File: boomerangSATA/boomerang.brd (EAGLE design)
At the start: 84.1 x 79.3 mm, 12 parts

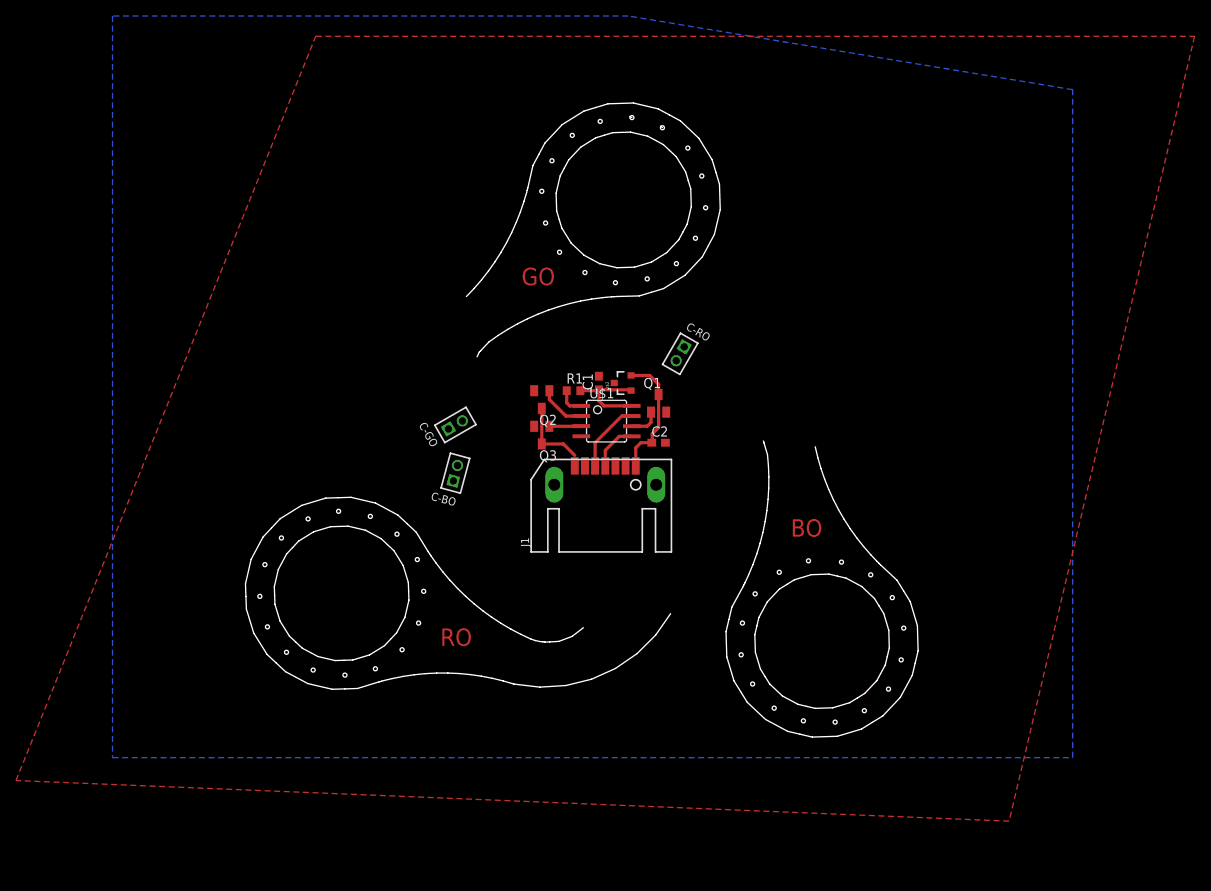
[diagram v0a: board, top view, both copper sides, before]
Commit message: foo
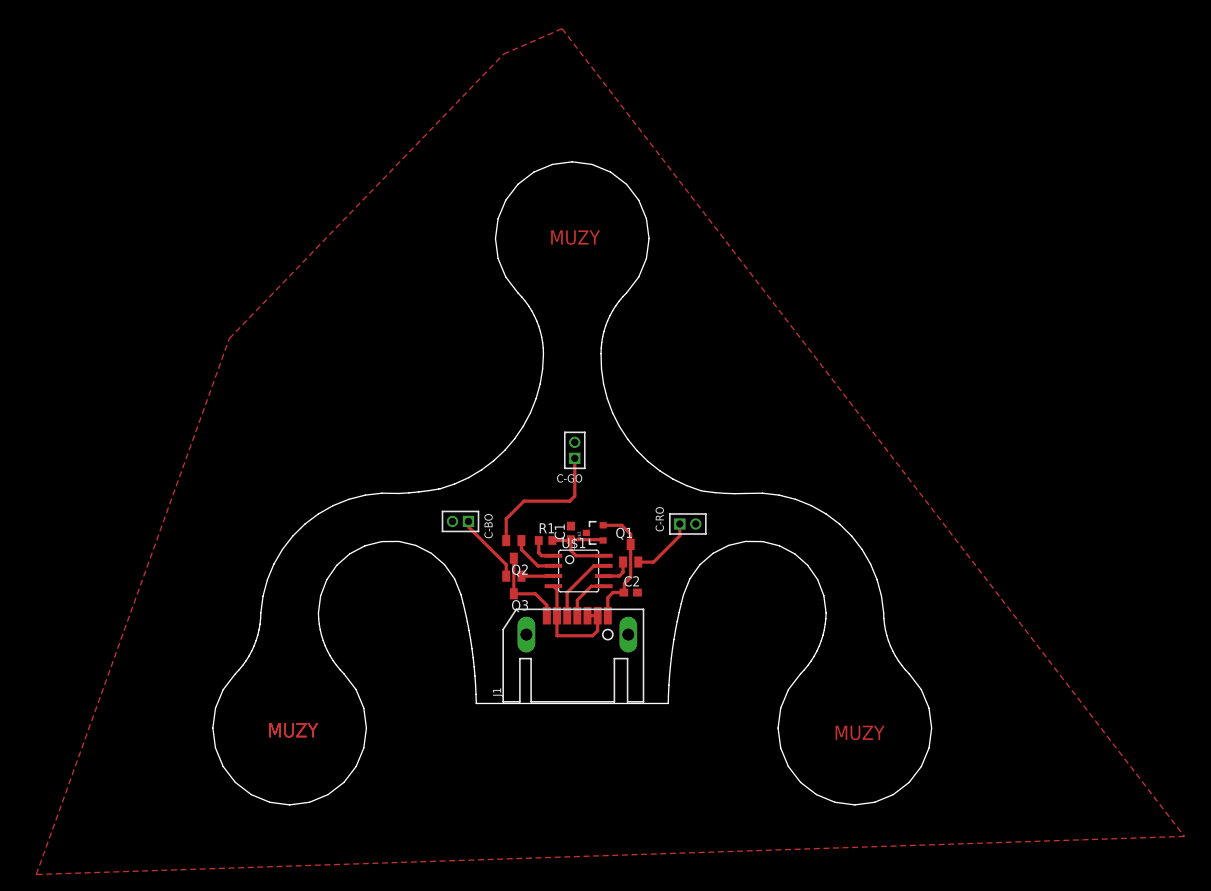
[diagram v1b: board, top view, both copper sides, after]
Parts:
- moved C-RO 21.3 mm to (14.4, -5.08), turned to 0 degrees
- moved C1 19.1 mm to (-0.16, -6.19)
- moved C2 19.1 mm to (7.30, -13.7)
- moved Q1 19.1 mm to (7.30, -8.73)
- moved Q2 19.1 mm to (-7.30, -8.26)
- moved U$2 19.1 mm to (2.86, -6.19)
- moved J1 19.1 mm to (0.64, -21.0)
- moved Q3 19.1 mm to (-7.30, -12.7)
- moved R1 19.1 mm to (-3.33, -7.14)
- moved U$1 19.1 mm to (0.79, -11.0)
- moved C-GO 15.3 mm to (0.32, 4.13), turned to 90 degrees
- moved C-BO 6.07 mm to (-14.0, -4.76), turned to 180 degrees
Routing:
- net GO: track 0.00 -> 17.2 mm
- net GND: track 0.00 -> 15.5 mm
- net BO: track 0.00 -> 8.86 mm
- net RO: track 0.00 -> 8.04 mm
- net VCC: track 25.3 -> 26.6 mm
- removed copper zone on layer 16, net GND
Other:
- board size 84.1 x 79.3 mm -> 89.8 x 80.4 mm
- board text added: "MUZY"
- board text removed: "BO"
- board text removed: "GO"
- board text removed: "RO"
